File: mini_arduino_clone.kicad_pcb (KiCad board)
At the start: 4 copper layers, 43.4 x 18 mm, 32 parts, among them J101 USB_B_Micro, J102 Conn_02x03_Odd_Even, J103 Conn_01x13, J104 Conn_01x13, SW101 SW_Push, U101 ATmega328P-AU, U201 XC6220B331MR-G, U301 CP2102-GMR, Y101 16MHz

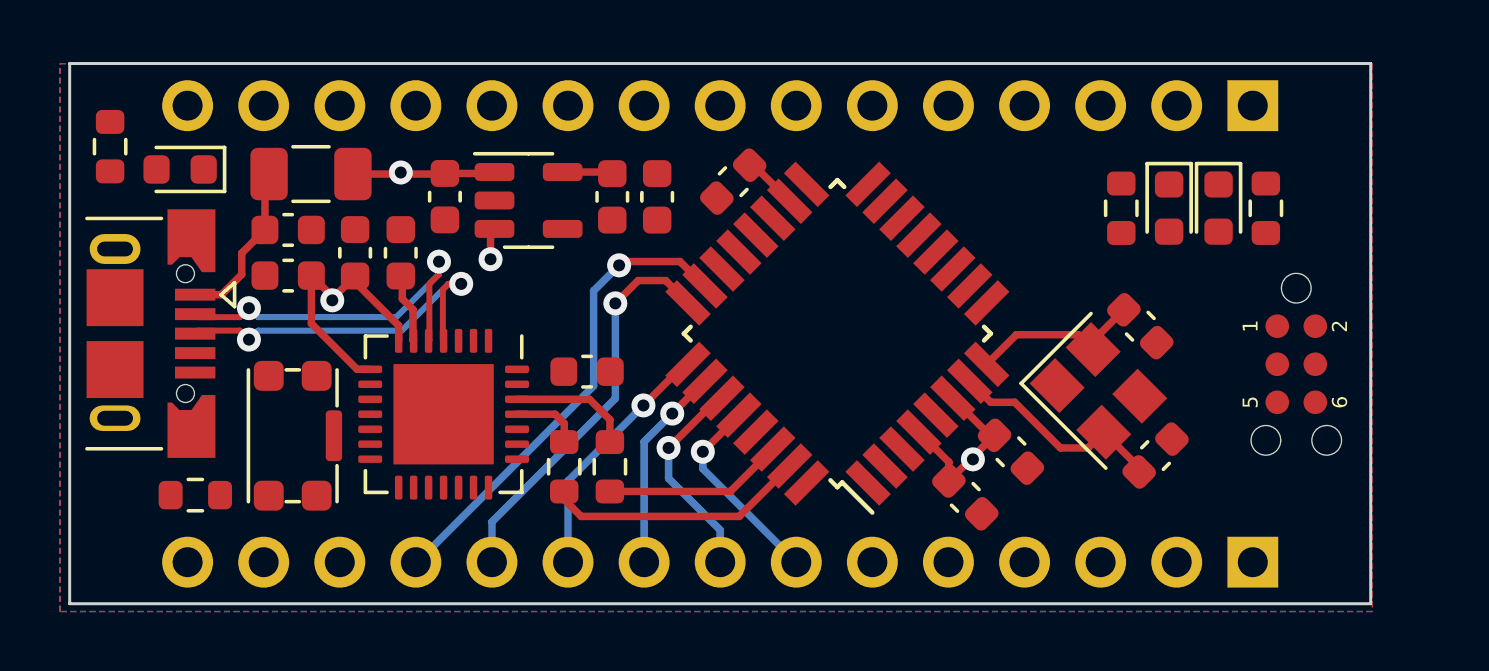
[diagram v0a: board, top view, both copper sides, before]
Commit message: update layout and schematics
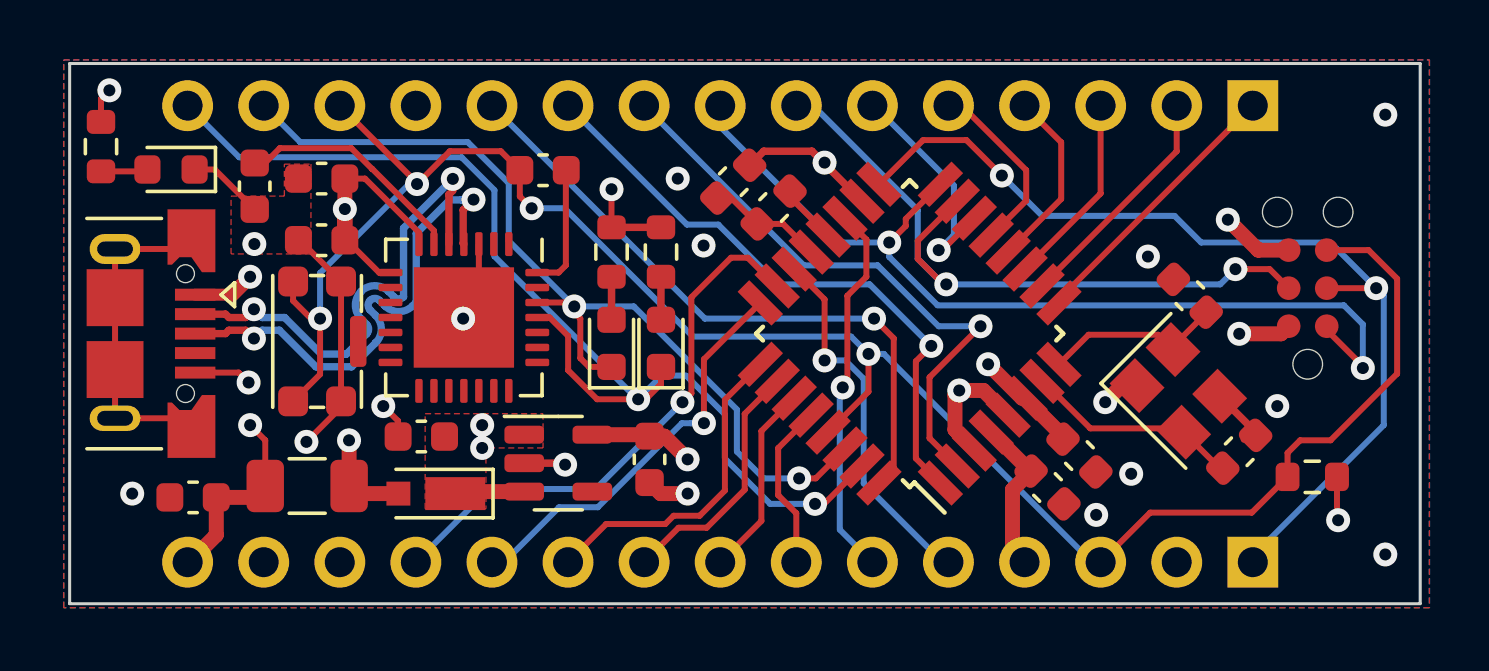
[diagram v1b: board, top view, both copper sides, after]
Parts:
- removed R101, R102: 1K, Resistor_SMD:R_0603_1608Metric
- added D1: MSS1P4, Diode_SMD:D_MicroSMP_AK, F.Cu at (80.4, 63.2)
- moved R103 37.3 mm to (109.9, 62.7), turned to 180 degrees
- moved R105 20.2 mm to (88.1, 55.2)
- moved D101 19.2 mm to (86.5, 58.2), turned to 90 degrees
- moved D102 19.2 mm to (88.1, 58.2), turned to 90 degrees
- moved R104 17.1 mm to (86.5, 55.2)
- moved F101 10.4 mm to (76.3, 63.0)
- moved C102 9.48 mm to (72.5, 63.4), turned to 180 degrees
- moved C202 8.85 mm to (87.8, 62.1)
- moved U201 8.83 mm to (84.7, 62.2)
- moved C201 8.05 mm to (80.1, 61.3), turned to 0 degrees
- moved C108 6.88 mm to (84.2, 52.5)
- moved C303 5.36 mm to (74.6, 53.0), turned to -90 degrees
- moved C101 3.90 mm to (91.9, 53.7), turned to -135 degrees
- moved U301 3.30 mm to (81.6, 57.4)
- moved SW101 3.25 mm to (76.7, 58.2)
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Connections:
- C301 pad 1: +5V -> /USB_UART/VBUS
- C302 pad 1: +5V -> /USB_UART/VBUS
- D101 pad 1: /RX -> /D0/RX
- D102 pad 1: /TX -> /D1/TX
- F101 pad 2: +5V -> /USB_UART/VBUS
- J102 pad 2: VBUS -> +5V
- J103 pad 1: /TX -> /D5
- J103 pad 10: /D7 -> /D3
- J103 pad 11: /D8 -> /D2
- J103 pad 12: /D9 -> GND
- J103 pad 13: /D10 -> /~{RESET}
- J103 pad 14: /D11/MOSI -> /D0/RX
- J103 pad 15: /D12/MISO -> /D1/TX
- J103 pad 2: /RX -> /D6
- J103 pad 3: /~{RESET} -> /D7
- J103 pad 4: GND -> /D8
- J103 pad 5: /D2 -> /D9
- J103 pad 6: /D3 -> /D10
- J103 pad 7: /D4 -> /D11/MOSI
- J103 pad 8: /D5 -> /D12/MISO
- J103 pad 9: /D6 -> /D4
- J104 pad 1: VBUS -> /D13/SCK
- J104 pad 13: /AREF -> GND
- J104 pad 15: /D13/SCK -> VBUS
- U101 pad 30: /RX -> /D0/RX
- U101 pad 31: /TX -> /D1/TX
- U301 pad 25: /TXD -> /D1/TX
- U301 pad 26: /RXD -> /D0/RX
- U301 pad 7: +5V -> /USB_UART/VBUS
- U301 pad 8: +5V -> /USB_UART/VBUS
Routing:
- net /~{RESET}: track 0.00 -> 66.1 mm, vias 0 -> 4
- net GND: track 0.00 -> 40.7 mm, vias 0 -> 19
- net /D1/TX: track 0.00 -> 38.1 mm, vias 0 -> 2
- net /D13/SCK: track 0.00 -> 32.0 mm, vias 0 -> 2
- net /D0/RX: track 0.00 -> 31.2 mm, vias 0 -> 2
- net /D12/MISO: track 0.00 -> 31.2 mm, vias 0 -> 2
- net /D11/MOSI: track 0.00 -> 24.1 mm, vias 0 -> 2
- net /D2: track 0.00 -> 21.7 mm, vias 0 -> 1
- net /D3: track 0.00 -> 20.6 mm, vias 0 -> 1
- net /D4: track 0.00 -> 20.0 mm, vias 0 -> 1
- net /USB_UART/VBUS: track 0.00 -> 19.7 mm, vias 0 -> 2
- net +3V3: track 1.78 -> 19.1 mm, vias 0 -> 1
- net /A6: track 0.00 -> 12.6 mm, vias 0 -> 1
- net /A7: track 0.00 -> 12.4 mm, vias 0 -> 1
- net unconnected-(J101-Shield-Pad6): track 0.00 -> 11.0 mm
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- added copper zone on F.Cu, net +5V
- added copper zone on In1.Cu, net VBUS
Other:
- board size 43.4 x 18 mm -> 45.1 x 18 mm
